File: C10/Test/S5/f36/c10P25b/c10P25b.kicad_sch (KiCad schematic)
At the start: 5 parts

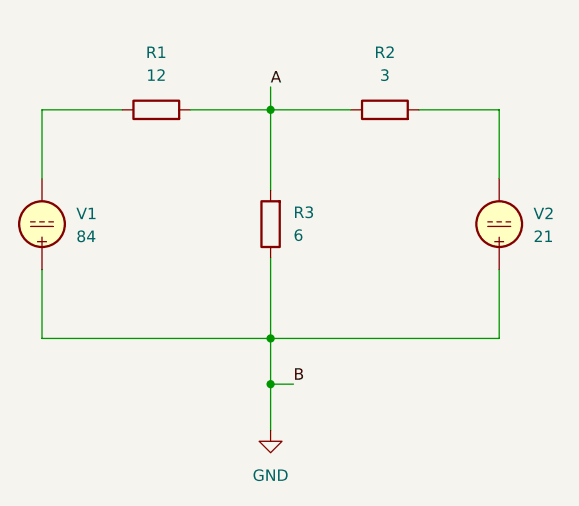
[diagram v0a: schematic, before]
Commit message: additiona upload Chapter 10
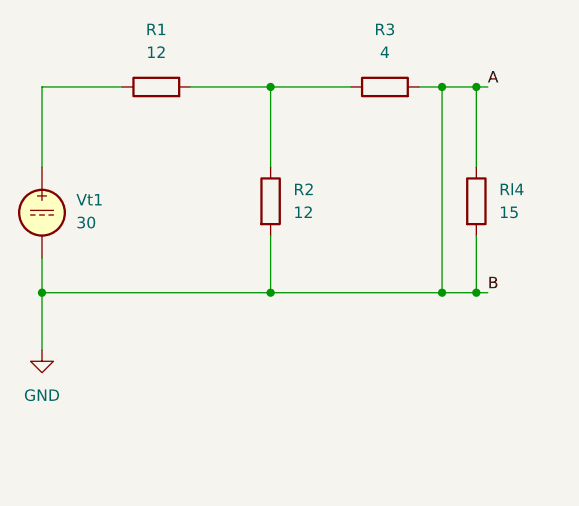
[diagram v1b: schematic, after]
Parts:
- removed V1: 84, symbol Simulation_SPICE:VDC
- removed V2: 21, symbol Simulation_SPICE:VDC
- added Rl4: 15, symbol Device:R
- added Vt1: 30, symbol Simulation_SPICE:VDC
- R2: value 3 -> 12
- R3: value 6 -> 4
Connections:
- net GND: now also R2.2, R3.2, Rl4.1, Rl4.2, Vt1.2; no longer R3.1
- net at R1.1: now also Vt1.1
- net A: no longer names the net of R1.2, R2.1
- net A: now also R3.1; no longer R3.2
